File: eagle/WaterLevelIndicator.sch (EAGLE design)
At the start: 7 parts, among them IC2 MAX7219CNG

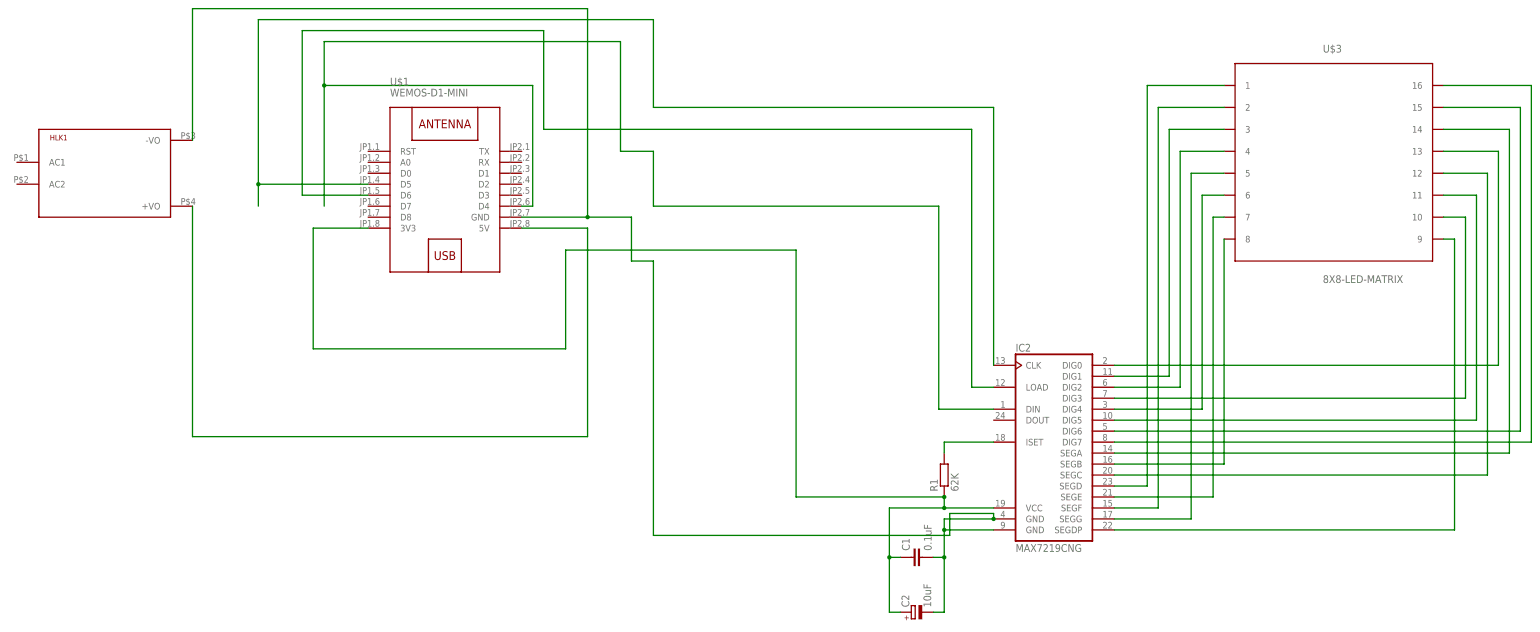
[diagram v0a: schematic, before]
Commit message: new board
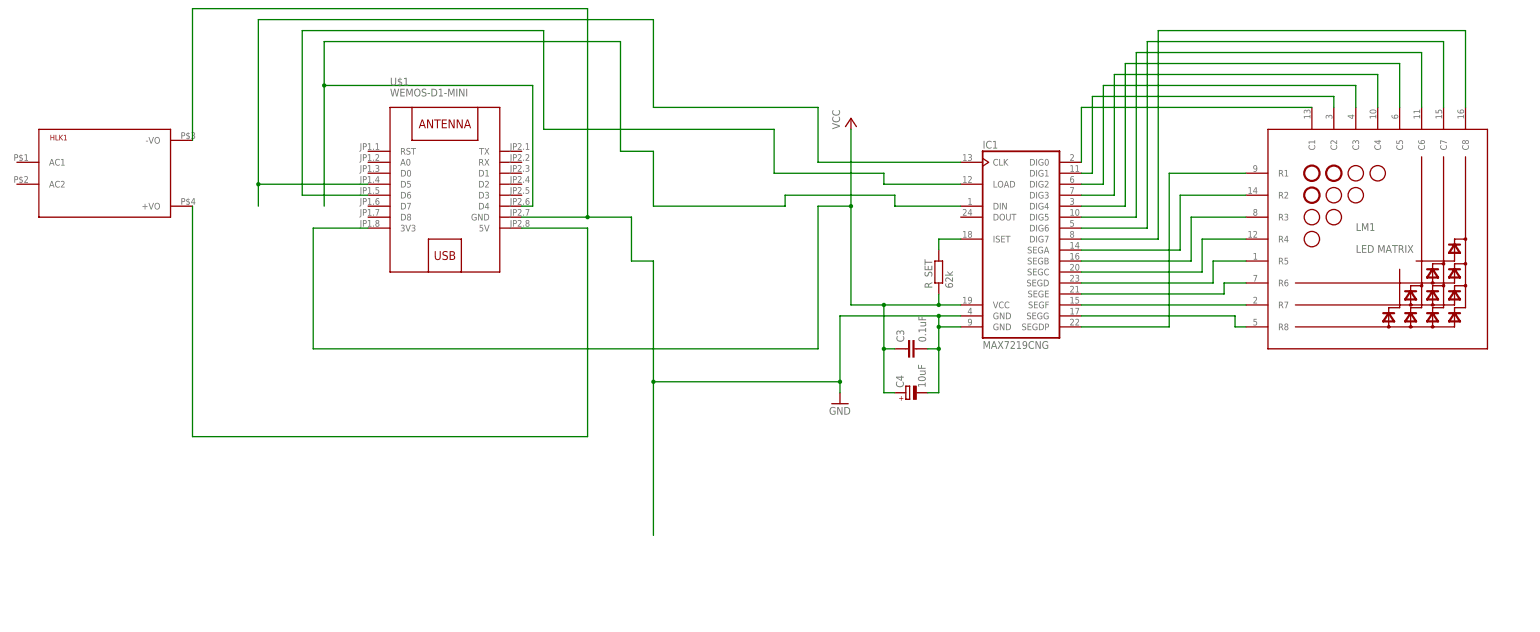
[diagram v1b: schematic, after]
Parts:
- removed C1: 0.1uF, rcl:C-EU025-024X044
- removed C2: 10uF, rcl:CPOL-EUE2-5
- removed IC2: MAX7219CNG, maxim:MAX7219CNG
- removed R1: 62K, resistor:R-EU_0207/10
- removed U$3: 8X8-LED-MATRIX, 8 X 8 LED Matrix:8X8-LED-MATRIX
- added C3: 0.1uF, rcl:C-EU025-024X044
- added C4: 10uF, rcl:CPOL-EUE2-5
- added IC1: MAX7219CNG, maxim:MAX7219CNG
- added LM1: LED MATRIX, MajicDesigns:LD-1088BS_LED_MATRIX
- added R_SET: 62k, rcl:R-EU_0207/10
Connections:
- removed net N$1: C1.2, C2.-, HLK1.-VO, IC2.GND@1, IC2.GND@2, U$1.GND
- removed net N$12: IC2.DIG0, U$3.13
- removed net N$13: IC2.DIG1, U$3.3
- removed net N$14: IC2.DIG2, U$3.4
- removed net N$15: IC2.DIG3, U$3.10
- removed net N$16: IC2.DIG4, U$3.6
- removed net N$17: IC2.DIG5, U$3.11
- removed net N$18: IC2.DIG6, U$3.15
- removed net N$19: IC2.DIG7, U$3.16
- removed net N$20: IC2.SEGA, U$3.14
- removed net N$21: IC2.SEGB, U$3.8
- removed net N$22: IC2.SEGC, U$3.12
- removed net N$23: IC2.SEGD, U$3.1
- removed net N$24: IC2.SEGE, U$3.7
- removed net N$25: IC2.SEGF, U$3.2
- removed net N$26: IC2.SEGG, U$3.5
- removed net N$27: IC2.SEGDP, U$3.9
- removed net N$28: C1.1, C2.+, IC2.VCC, R1.1, U$1.3V3
- removed net N$7: IC2.ISET, R1.2
- new net GND: C3.2, C4.-, HLK1.-VO, IC1.GND@1, IC1.GND@2, U$1.GND
- new net N$10: IC1.SEGC, LM1.R4
- new net N$11: IC1.SEGB, LM1.R3
- new net N$29: IC1.SEGA, LM1.R2
- new net N$3: IC1.SEGF, LM1.R7
- new net N$30: IC1.SEGDP, LM1.R1
- new net N$31: IC1.DIG7, LM1.C8
- new net N$32: IC1.DIG6, LM1.C7
- new net N$33: IC1.DIG5, LM1.C6
- new net N$34: IC1.DIG4, LM1.C5
- new net N$35: IC1.DIG3, LM1.C4
- new net N$36: IC1.DIG2, LM1.C3
- new net N$37: IC1.DIG1, LM1.C2
- new net N$38: IC1.DIG0, LM1.C1
- new net N$43: IC1.ISET, R_SET.2
- new net N$44: IC1.SEGG, LM1.R8
- new net N$8: IC1.SEGE, LM1.R6
- new net N$9: IC1.SEGD, LM1.R5
- new net VCC: C3.1, C4.+, IC1.VCC, R_SET.1, U$1.3V3
- net N$4: now also IC1.DIN; no longer IC2.DIN
- net N$5: now also IC1.LOAD; no longer IC2.LOAD
- net N$6: now also IC1.CLK; no longer IC2.CLK
